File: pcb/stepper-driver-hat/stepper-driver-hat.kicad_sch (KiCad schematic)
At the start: 5 parts, among them J1 Raspberry_Pi_4, U1 TMC2208_SILENTSTEPSTICK, U2 TMC2208_SILENTSTEPSTICK

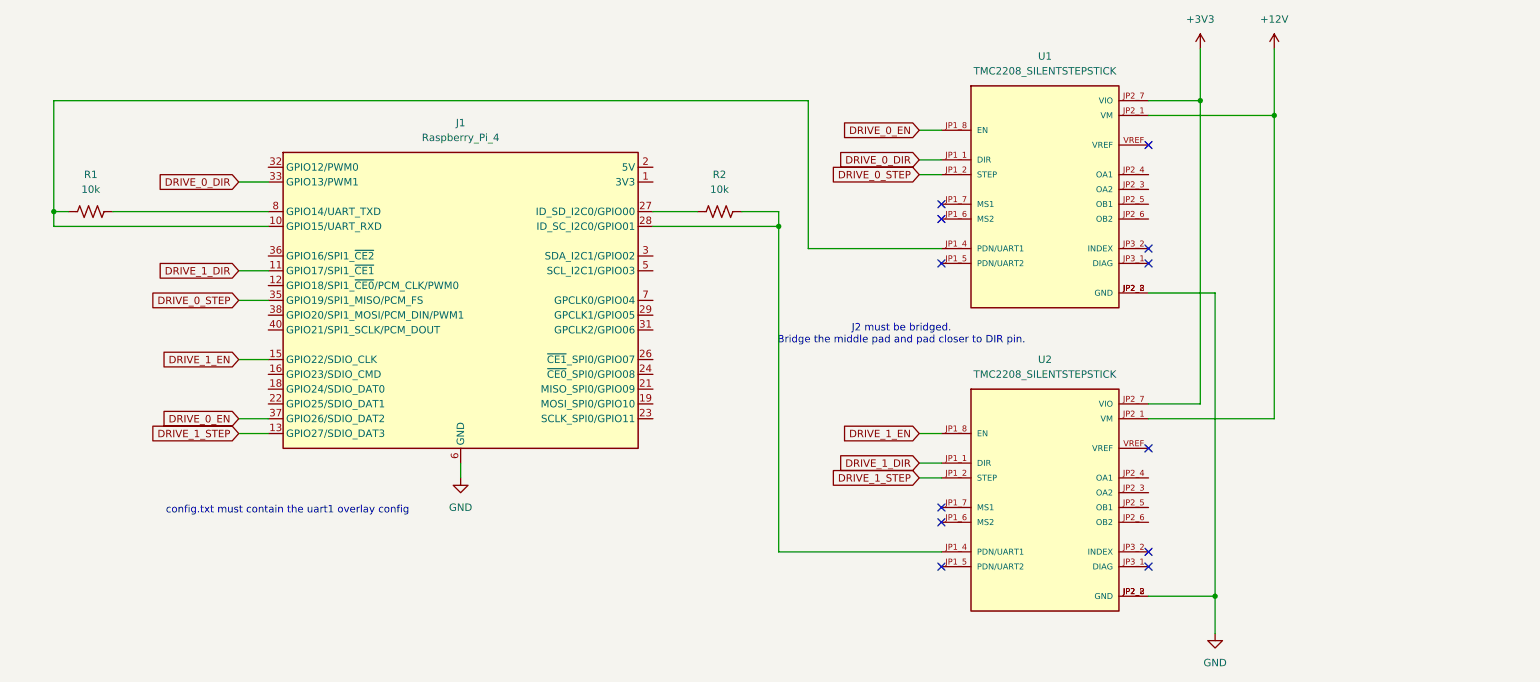
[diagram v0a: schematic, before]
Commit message: esp32 comm started
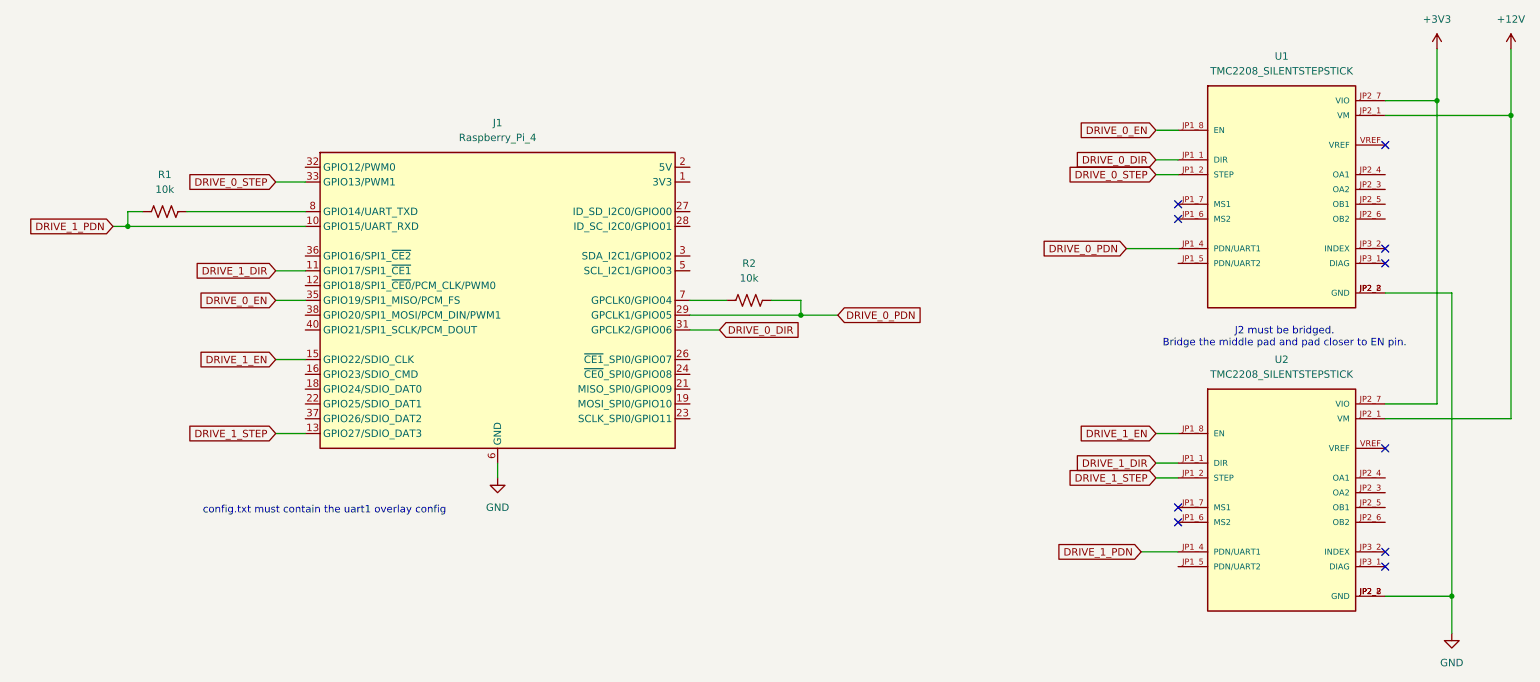
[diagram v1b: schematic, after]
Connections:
- net DRIVE_0_DIR: now also J1.31 (GPCLK2/GPIO06); no longer J1.33 (GPIO13/PWM1)
- net DRIVE_0_EN: now also J1.35 (GPIO19/SPI1_MISO/PCM_FS); no longer J1.37 (GPIO26/SDIO_DAT2)
- net DRIVE_0_STEP: now also J1.33 (GPIO13/PWM1); no longer J1.35 (GPIO19/SPI1_MISO/PCM_FS)
- net at R2.1: now also J1.7 (GPCLK0/GPIO04); no longer J1.27 (ID_SD_I2C0/GPIO00)
- net DRIVE_1_PDN: now reaches J1.10 (GPIO15/UART_RXD), R1.1
- net DRIVE_1_PDN: now also U2.JP1_4 (PDN/UART1); no longer U1.JP1_4 (PDN/UART1)
- net DRIVE_0_PDN: now reaches J1.29 (GPCLK1/GPIO05)
- net DRIVE_0_PDN: now also R2.2, U1.JP1_4 (PDN/UART1)
- now unconnected: J1.28 (ID_SC_I2C0/GPIO01)
- no-connect marks 12 -> 10
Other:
- note added: "J2 must be bridged. Bridge the middle pad and pad closer to EN pin."
- note removed: "J2 must be bridged. Bridge the middle pad and pad closer to DIR pin."
- moved on the sheet: J1, R1, R2, U1, U2
